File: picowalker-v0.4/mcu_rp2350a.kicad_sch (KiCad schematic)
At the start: 26 parts, among them SW1 ~{BOOT}, SW2 RUN, U1 RP2350A-QFN60, Y1 ABM8-272-T3

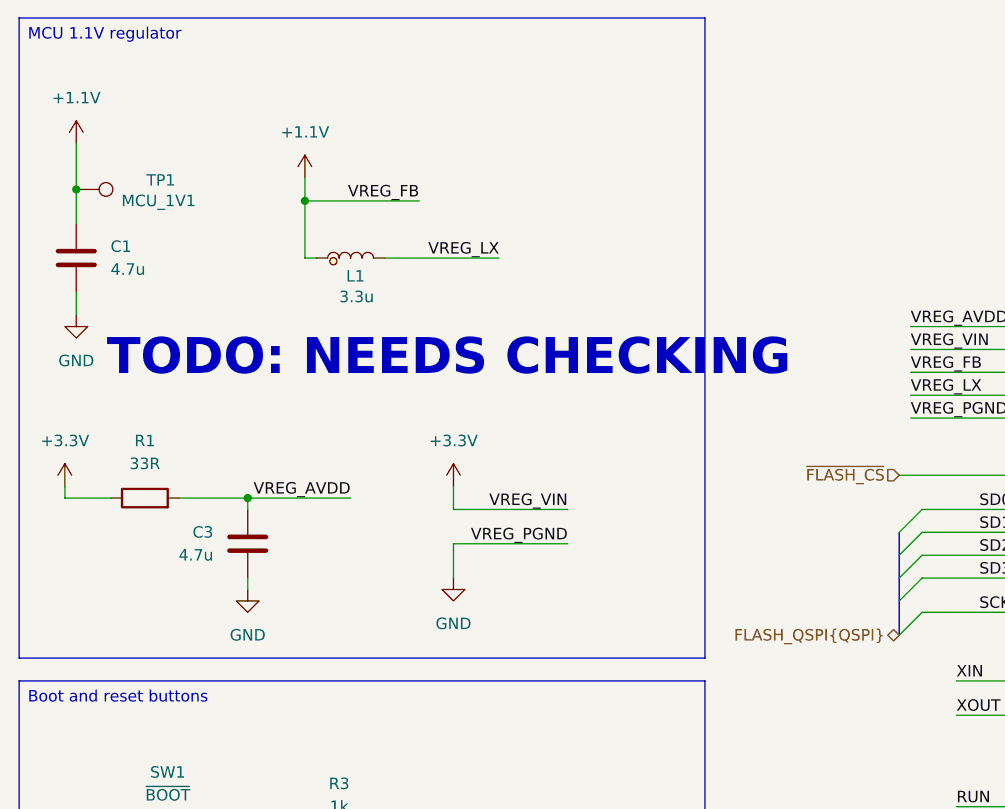
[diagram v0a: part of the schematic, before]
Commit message: v0.4: more rationalisation
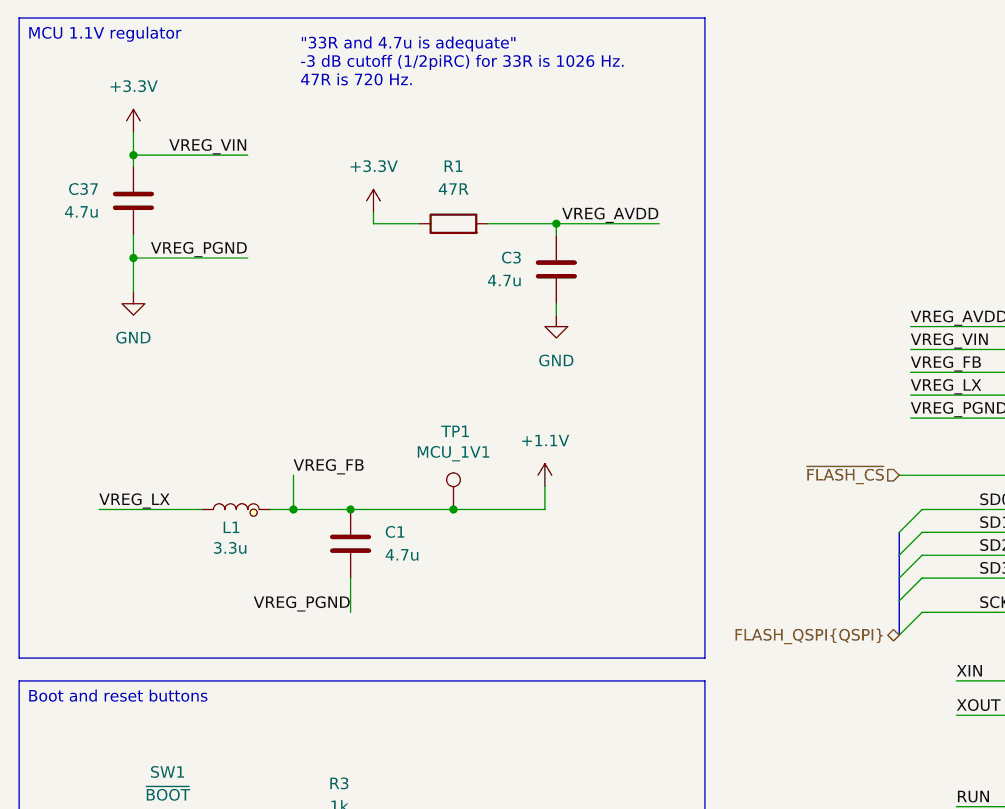
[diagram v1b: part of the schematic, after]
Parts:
- added C37: 4.7u, Capacitor_SMD:C_0402_1005Metric, symbol Device:C
- R1: value 33R -> 47R
- TP1: now left out of the parts list
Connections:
- net +3.3V: now also C37.1
- net GND: now also C37.2
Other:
- note added: ""33R and 4.7u is adequate" -3 dB cutoff (1/2piRC) for 33R is 1026 Hz. 47R is 720 Hz."
- note removed: "TODO: NEEDS CHECKING"
- moved on the sheet: C1, C3, L1, R1, TP1
